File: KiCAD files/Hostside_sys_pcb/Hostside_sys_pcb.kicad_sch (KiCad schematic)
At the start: 8 parts, among them U1 L7805, U2 Pico

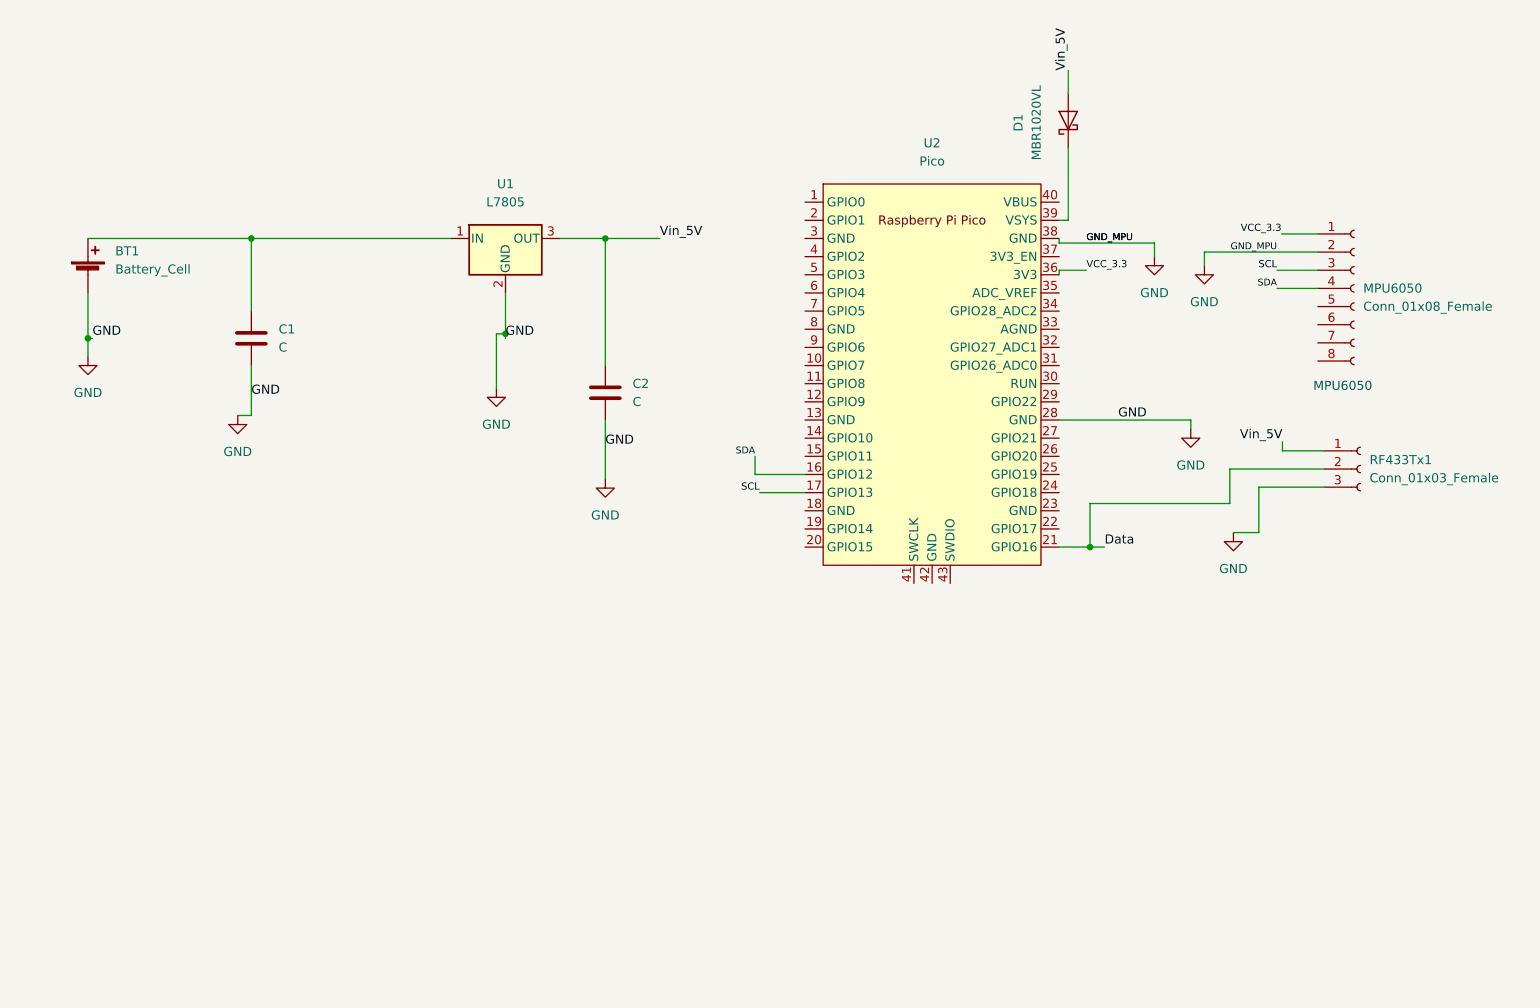
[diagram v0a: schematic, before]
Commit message: edited oops
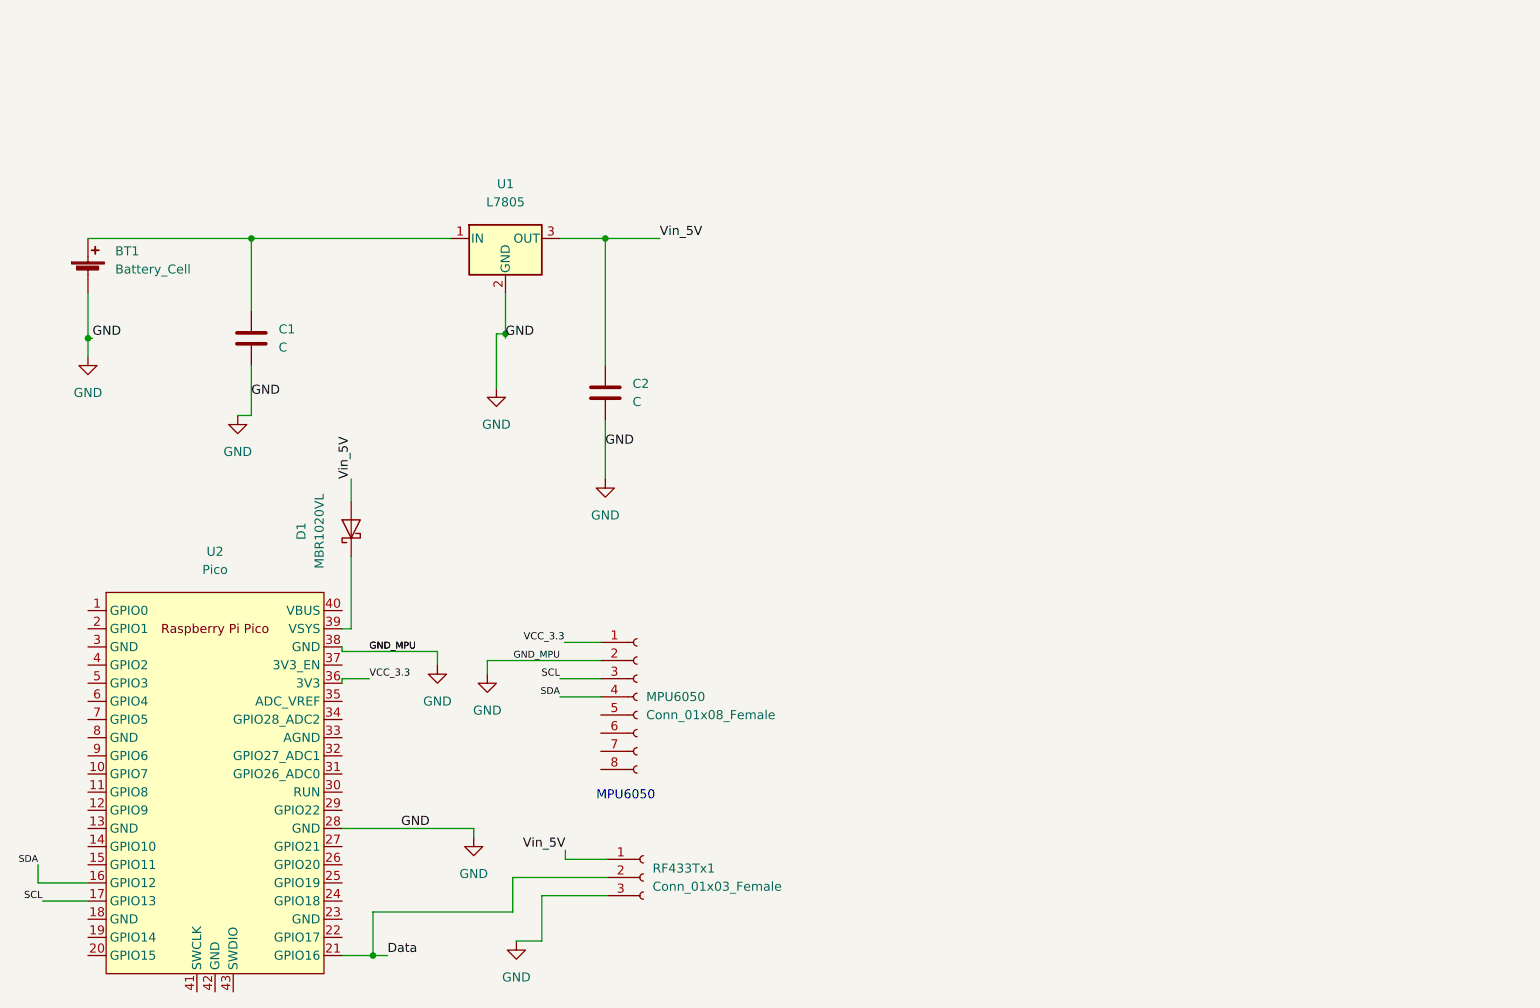
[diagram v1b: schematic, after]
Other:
- moved on the sheet: D1, MPU6050, RF433Tx1, U2
